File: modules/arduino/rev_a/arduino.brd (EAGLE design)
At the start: 67.3 x 66.7 mm, 58 parts, among them J1 MODULE_GENERIC, J3 ICSP_PROG, J4 MICRO_USB_B_HIROSE_ZX62-B-5PA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, J6 ICSP, U1 ADG3304, U2 ADG3304, U3 ATMEGA8U2-MU, U4 ATMEGA328P-20MU, U5 74LVC2G00DC, U6 SN74LVC1G123DCUR, Y1 12 MHz, Y2 16MHz

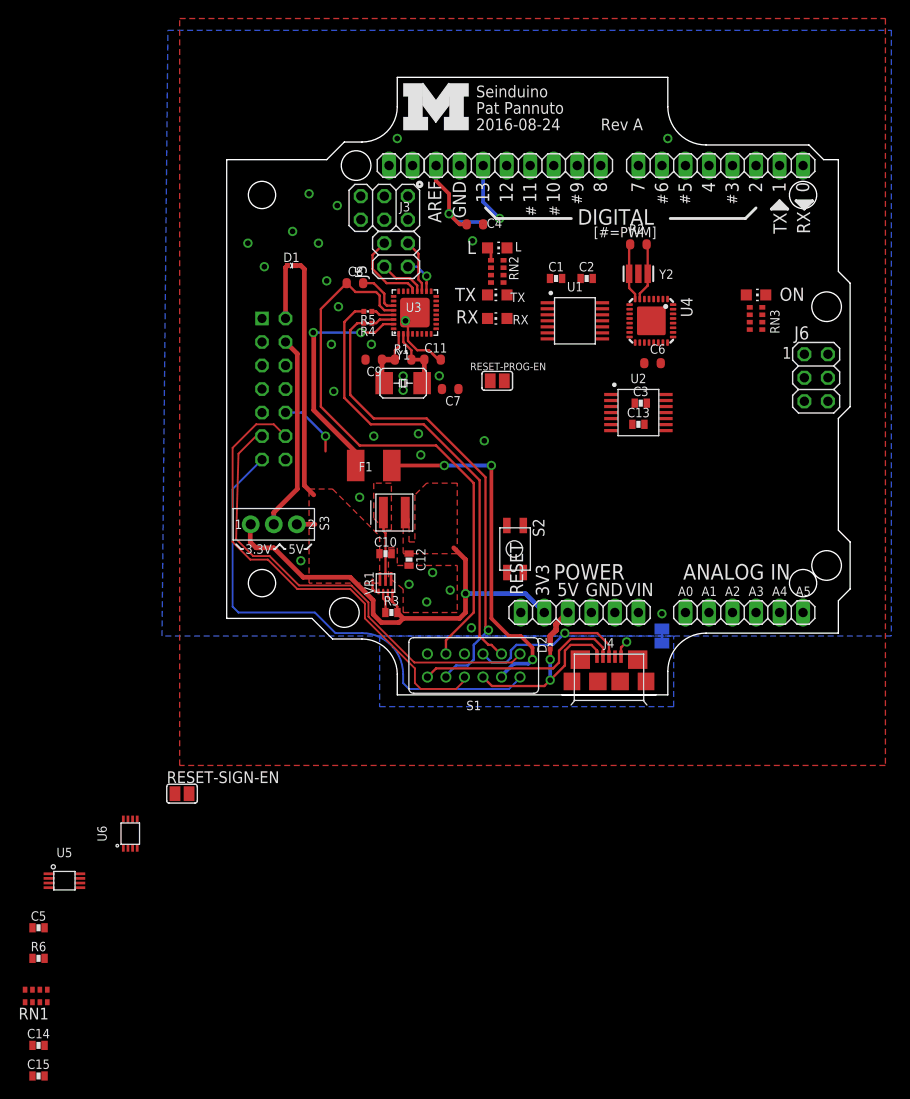
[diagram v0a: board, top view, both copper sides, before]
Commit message: Seinduino routed
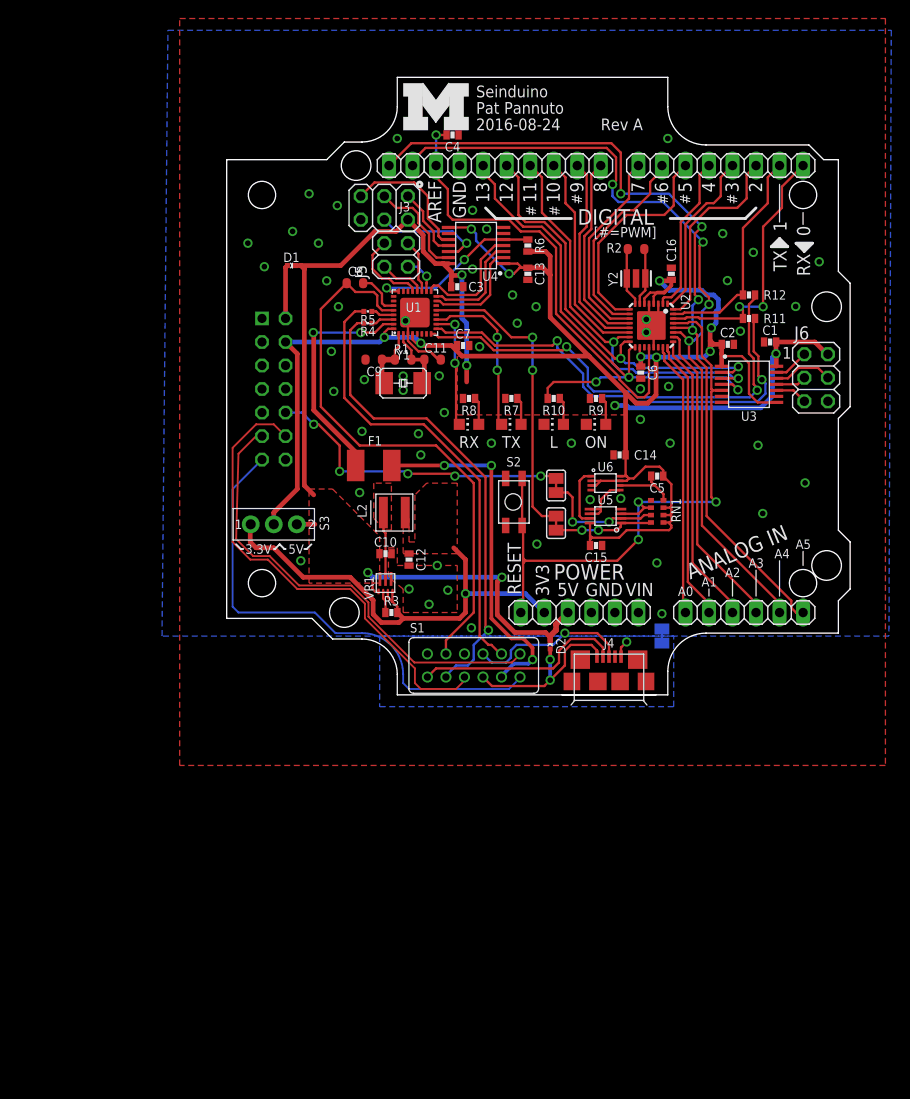
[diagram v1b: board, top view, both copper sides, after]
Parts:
- removed RN2, RN3: 1K, resistor-dil:CAY16
- added C16: 100nF, passives:0603_CAP
- added R10, R11, R12, R7, R8: 1kΩ, passives:0603-RES
- added R9: 470Ω, passives:0603-RES
- C4, C6: value 100n -> 100nF; device SmartPrj:C0603-ROUND -> passives:0603_CAP
- C7: device SmartPrj:C0603-ROUND -> passives:0603_CAP
- U1: value ADG3304 -> ATMEGA8U2-MU; device chips:TSSOP-14/5MM -> atmel:QFN32
- U2: value ADG3304 -> ATMEGA328P-20MU; device chips:TSSOP-14/5MM -> idii:MLF32
- U3: value ATMEGA8U2-MU -> ADG3304; device atmel:QFN32 -> chips:TSSOP-14/5MM
- U4: value ATMEGA328P-20MU -> ADG3304; device idii:MLF32 -> chips:TSSOP-14/5MM
- moved R6 93.4 mm to (33.8, 42.2), turned to 270 degrees
- moved C14 89.4 mm to (43.7, 19.6)
- moved RN1 85.1 mm to (47.8, 13.5), turned to 90 degrees
- moved C15 83.1 mm to (41.1, 9.78), turned to 180 degrees
- moved C5 82.7 mm to (47.8, 17.3), turned to 180 degrees
- moved U5 70.4 mm to (42.2, 13.0), turned to 180 degrees
- moved U6 63.8 mm to (42.2, 16.5), turned to 270 degrees
- moved RESET-SIGN-EN 52.3 mm to (36.8, 16.3), turned to 90 degrees
- moved U3 36.9 mm to (57.7, 27.2), turned to 0 degrees
- moved C1 24.1 mm to (59.9, 31.8), turned to 180 degrees
- moved C3 23.5 mm to (26.2, 37.7)
- moved ON 22.2 mm to (41.1, 22.9), turned to 90 degrees
- moved U4 20.6 mm to (28.2, 42.2), turned to 180 degrees
- moved C13 20.2 mm to (33.8, 39.1), turned to 90 degrees
- moved L 20.0 mm to (36.6, 22.9), turned to 90 degrees
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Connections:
- removed net N$10: RESET-SIGN-EN.2, RN1.7, U5.2
- removed net N$9: RESET-PROG-EN.2, RN1.8, U5.1
- net +5V: now also R7.2, R8.2, R9.1, U3.14, U4.14; no longer RN2.2, RN2.3, RN3.3, RN3.4, U1.14, U2.14
- net AD0: now also U2.23; no longer U4.23
- net AD1: now also U2.24; no longer U4.24
- net AD2: now also U2.25; no longer U4.25
- net AD3: now also U2.26; no longer U4.26
- net AD4: now also U2.27; no longer U4.27
- net AD5: now also U2.28; no longer U4.28
- net ARD_USB_D+_TERM: now also U1.29; no longer U3.29
- net ARD_USB_D-_TERM: now also U1.30; no longer U3.30
- net ARD_USB_GND: now also U1.28; no longer U3.28
- net AREF: now also U2.20; no longer U4.20
- net DTR_PROG: now also RESET-PROG-EN.2, RN1.8, U1.13, U5.1; no longer U3.13
- net GND: now also C16.2, C6.2, RN1.5, U1.3, U1.EXP, U2.21, U2.3, U2.5, U3.7, U4.7; no longer C6.1, RN1.6, U1.7, U2.7, U3.3, U3.EXP, U4.21, U4.3, U4.5
- net IO0: now also R11.2, U2.30; no longer RN3.2, U4.30
- net IO1: now also R12.2, U2.31; no longer RN3.1, U4.31
- net IO2: now also U2.32; no longer U4.32
- net IO3: now also U2.1; no longer U4.1
- net IO4: now also U2.2; no longer U4.2
- net IO5: now also U2.9; no longer U4.9
- net IO6: now also U2.10; no longer U4.10
- net IO7: now also U2.11; no longer U4.11
- net IO8: now also U2.12; no longer U4.12
- net IO9: now also U2.13; no longer U4.13
- net M8RXD: now also R11.1, U1.9; no longer RN3.7, U3.9
- net M8TXD: now also R12.1, U1.8; no longer RN3.8, U3.8
- net MISO: now also U2.16, U3.2; no longer U2.2, U4.16
- net MISO_PROG: now also U1.17, U4.4; no longer U1.2, U3.17
- net MISO_PROG_SHIFTED: now also U4.11; no longer U1.13
- net MISO_SHIFTED: now also U3.13; no longer U2.13
- net MOD_IN: now also RESET-SIGN-EN.2, RN1.7, U5.2
- net MOSI: now also U2.15, U3.3; no longer U2.3, U4.15
- net MOSI_PROG: now also U1.16, U4.3; no longer U1.3, U3.16
- net MOSI_PROG_SHIFTED: now also U4.12; no longer U1.12
- net MOSI_SHIFTED: now also U3.12; no longer U2.12
- net N$1: now also R10.2; no longer RN2.1
- net N$2: now also U1.18; no longer U3.18
- net N$3: now also R9.2; no longer RN3.5, RN3.6
- net N$35: now also R8.1; no longer RN2.7
- net N$36: now also R7.1; no longer RN2.6
- net N$4: now also U1.19; no longer U3.19
- net N$5: now also U1.20; no longer U3.20
- net N$6: now also U1.21; no longer U3.21
- net N$7: now also RN1.4; no longer RN1.3
- net RESET: now also RN1.6, U2.29, U3.5; no longer RN1.5, U2.5, U4.29
- net RESET_PROG: now also U1.24, U4.5; no longer U1.5, U3.24
- net RESET_PROG_SHIFTED: now also U4.10; no longer U1.10
- net RESET_SHIFTED: now also U3.10; no longer U2.10
- net RXLED: now also U1.10; no longer U3.10
- net SCK: now also R10.1, U2.17, U3.4; no longer RN2.8, U2.4, U4.17
- net SCK_PROG: now also U1.15, U4.2; no longer U1.4, U3.15
- net SCK_PROG_SHIFTED: now also U4.13; no longer U1.11
- net SCK_SHIFTED: now also U3.11; no longer U2.11
- net SS: now also U2.14; no longer U4.14
- net TXLED: now also U1.11; no longer U3.11
- net USBVCC: now also U1.31; no longer U3.31
- net VCC: now also C16.1, C6.1, RN1.3, U1.32, U1.4, U2.18, U2.4, U2.6, U3.1, U3.8, U4.1, U4.8; no longer C6.2, RN1.4, U1.1, U1.8, U2.1, U2.8, U3.32, U3.4, U4.18, U4.4, U4.6
- net VUCAP: now also U1.27; no longer U3.27
- net XT1: now also U1.1; no longer U3.1
- net XT2: now also U1.2; no longer U3.2
- net XTAL1: now also U2.7; no longer U4.7
- net XTAL2: now also U2.8; no longer U4.8
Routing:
- net VCC: track 21.3 -> 190.9 mm, vias 0 -> 9
- net +5V: track 33.5 -> 127.4 mm, vias 0 -> 6
- net AD5: track 0.63 -> 91.1 mm, vias 0 -> 4
- net AD4: track 0.00 -> 87.6 mm, vias 0 -> 4
- net RESET: track 0.00 -> 69.5 mm, vias 0 -> 3
- net SCK: track 6.45 -> 59.1 mm, vias 1 -> 3
- net M8TXD: track 0.00 -> 50.7 mm, vias 0 -> 2
- net M8RXD: track 0.00 -> 49.6 mm, vias 0 -> 2
- net MISO: track 0.00 -> 45.2 mm, vias 0 -> 2
- net DTR_PROG: track 0.00 -> 45.2 mm, vias 0 -> 4
- net MOSI: track 0.00 -> 43.7 mm, vias 0 -> 2
- net MOD_IN: track 7.02 -> 48.8 mm, vias 1 -> 7
- net AREF: track 12.5 -> 49.6 mm
- net AD3: track 0.00 -> 33.7 mm
- net AD2: track 0.00 -> 31.9 mm
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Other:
- board text added: "Note: Pad connects to ground, but this part from Arduino neglects that, and they do not provide lbrs so cannot fix :("
- board text removed: "L"
